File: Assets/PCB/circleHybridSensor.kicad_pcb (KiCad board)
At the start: 2 copper layers, 40.6 x 40.6 mm, 24 parts, among them IC1 MCP23017ML, U4 MPU-6050, j2 R_0805_2012Metric

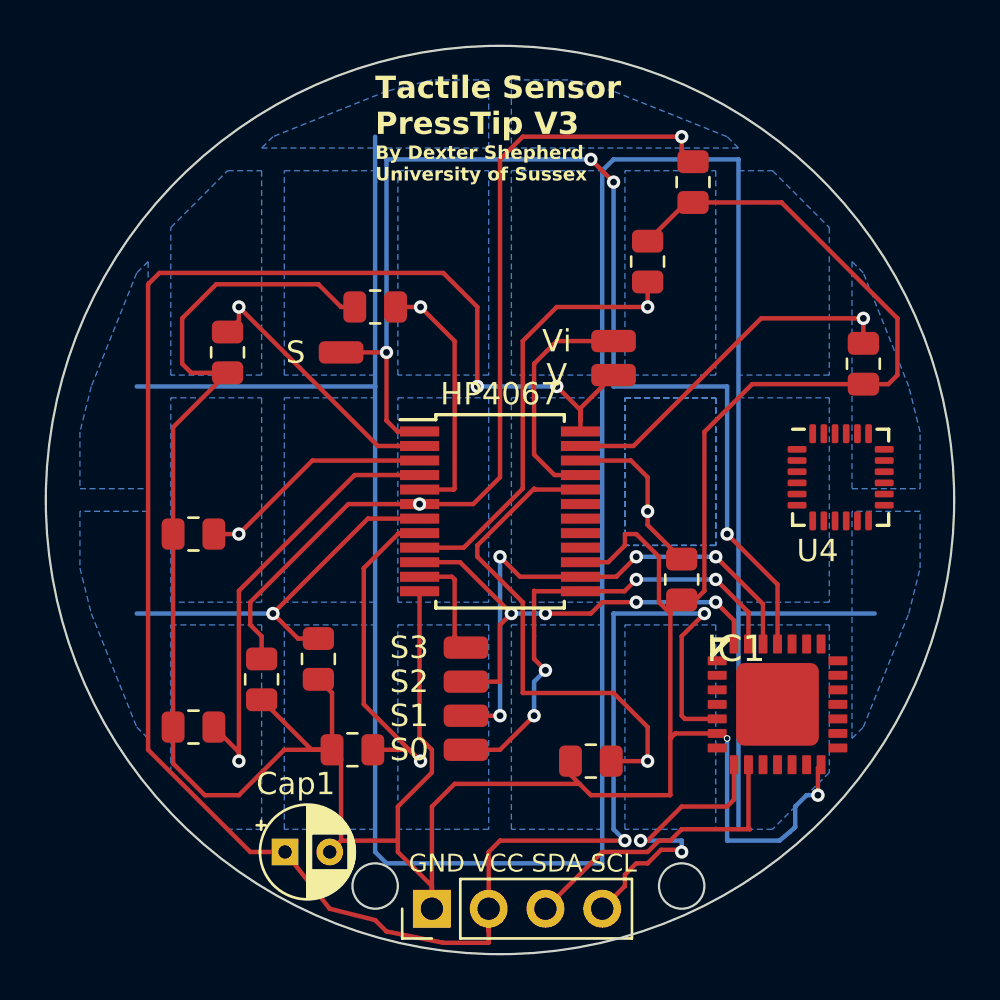
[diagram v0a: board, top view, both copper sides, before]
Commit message: Update circleHybridSensor.kicad_pcb
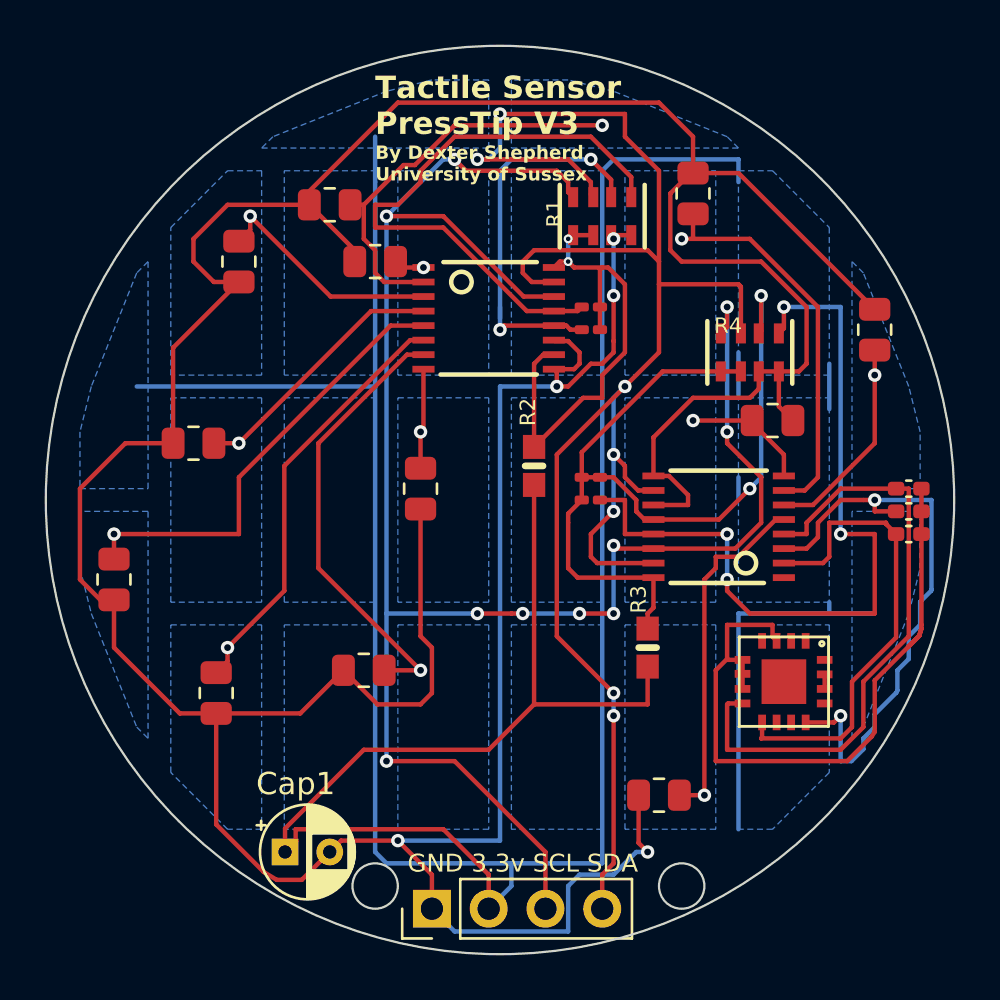
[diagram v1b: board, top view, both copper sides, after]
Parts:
- removed HP4067: SSOP-24_5.3x8.2mm_P0.65mm, Package_SO:SSOP-24_5.3x8.2mm_P0.65mm
- removed the IC1 at (164.8, 110.7)
- removed S, S0, S1, S2, S3, V, Vi: SolderWirePad_1x01_SMD_1x2mm, Connector_Wire:SolderWirePad_1x01_SMD_1x2mm
- removed U4: MPU-6050, Sensor_Motion:InvenSense_QFN-24_4x4mm_P0.5mm
- removed the j2 at (140.2, 95.0)
- removed the j2 at (146.8, 93.0)
- removed the j2 at (159.0, 90.9)
- removed the j2 at (138.7, 103.1)
- removed the j2 at (168.7, 95.5)
- removed the j2 at (160.5, 105.2)
- removed the j2 at (161.0, 87.4)
- removed the j2 at (144.3, 108.7)
- removed the j2 at (145.8, 112.8)
- removed the j2 at (141.7, 109.6)
- removed the j2 at (138.7, 111.8)
- removed the j2 at (156.5, 113.3)
- added C1: C_0402_1005Metric_Pad0.74x0.62mm_HandSolder, Capacitor_SMD:C_0402_1005Metric_Pad0.74x0.62mm_HandSolder, F.Cu at (170.7, 101.1)
- added C2: C_0402_1005Metric_Pad0.74x0.62mm_HandSolder, Capacitor_SMD:C_0402_1005Metric_Pad0.74x0.62mm_HandSolder, F.Cu at (170.7, 102.1)
- added C3: C_0402_1005Metric_Pad0.74x0.62mm_HandSolder, Capacitor_SMD:C_0402_1005Metric_Pad0.74x0.62mm_HandSolder, F.Cu at (170.7, 103.1)
- added IC1: ADC_ADS7830, TSSOP16, F.Cu at (162.2, 102.8)
- added IC1: ADC_ADS7830, TSSOP16, F.Cu at (151.9, 93.5)
- added IC1: ADXL33X, 16LCSP, F.Cu at (165.1, 109.7)
- added P1: C_0201_0603Metric_Pad0.64x0.40mm_HandSolder, Capacitor_SMD:C_0201_0603Metric_Pad0.64x0.40mm_HandSolder, F.Cu at (156.5, 93.0)
- added P2: C_0201_0603Metric_Pad0.64x0.40mm_HandSolder, Capacitor_SMD:C_0201_0603Metric_Pad0.64x0.40mm_HandSolder, F.Cu at (156.5, 94.0)
- added P3: C_0201_0603Metric_Pad0.64x0.40mm_HandSolder, Capacitor_SMD:C_0201_0603Metric_Pad0.64x0.40mm_HandSolder, F.Cu at (156.5, 101.6)
- added P4: C_0201_0603Metric_Pad0.64x0.40mm_HandSolder, Capacitor_SMD:C_0201_0603Metric_Pad0.64x0.40mm_HandSolder, F.Cu at (156.5, 100.6)
- added R1: 10K Pack, RESPACK_4X0603, F.Cu at (157.0, 88.9)
- added R2: 5ohm, 0603-NO, F.Cu at (153.9, 100.1)
- added R3: 5ohm, 0603-NO, F.Cu at (159.0, 108.2)
- added R4: 10K Pack, RESPACK_4X0603, F.Cu at (163.6, 95.0)
- added j0: R_0805_2012Metric, Resistor_SMD:R_0805_2012Metric, F.Cu at (139.7, 110.2)
- added j11: R_0805_2012Metric, Resistor_SMD:R_0805_2012Metric, F.Cu at (146.8, 90.9)
- added j2: R_0805_2012Metric, Resistor_SMD:R_0805_2012Metric, F.Cu at (138.7, 99.1)
- added j3: R_0805_2012Metric, Resistor_SMD:R_0805_2012Metric, F.Cu at (140.7, 90.9)
- added j7: R_0805_2012Metric, Resistor_SMD:R_0805_2012Metric, F.Cu at (148.8, 101.1)
- added j7: R_0805_2012Metric, Resistor_SMD:R_0805_2012Metric, F.Cu at (161.0, 87.9)
- added j7: R_0805_2012Metric, Resistor_SMD:R_0805_2012Metric, F.Cu at (146.3, 109.2)
- added j7: R_0805_2012Metric, Resistor_SMD:R_0805_2012Metric, F.Cu at (135.1, 105.2)
- added j7: R_0805_2012Metric, Resistor_SMD:R_0805_2012Metric, F.Cu at (159.5, 114.8)
- added j7: R_0805_2012Metric, Resistor_SMD:R_0805_2012Metric, F.Cu at (144.8, 88.4)
- added j8: R_0805_2012Metric, Resistor_SMD:R_0805_2012Metric, F.Cu at (164.6, 98.0)
- added j9: R_0805_2012Metric, Resistor_SMD:R_0805_2012Metric, F.Cu at (169.2, 94.0)
- GND 3.3v SCL SDA: renamed from GND VCC SDA SCL
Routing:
- net (no net): track 721.6 -> 931.5 mm, vias 36 -> 46
